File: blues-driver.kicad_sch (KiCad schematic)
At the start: 79 parts, among them Q1 LS844, Q10 BC848C, Q6 BC858C, Q7 LS844, Q8 BC858C, Q9 BC848C, U3 TLV9352

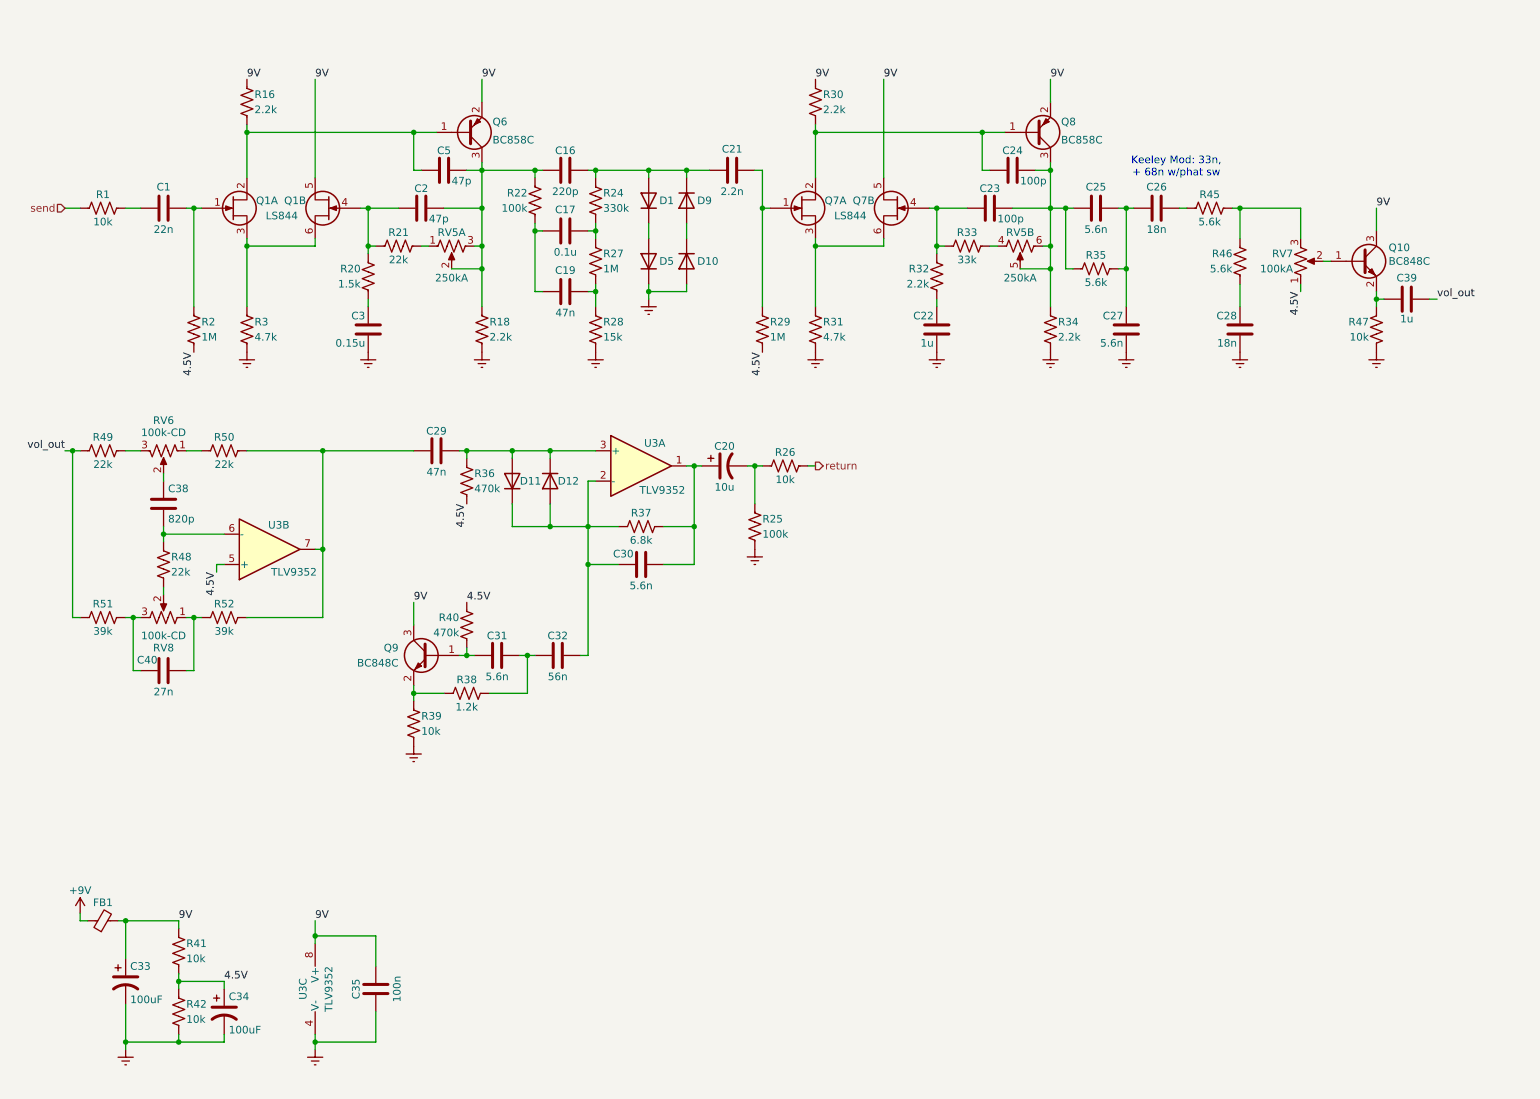
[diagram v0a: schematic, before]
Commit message: finished bd2 schematic
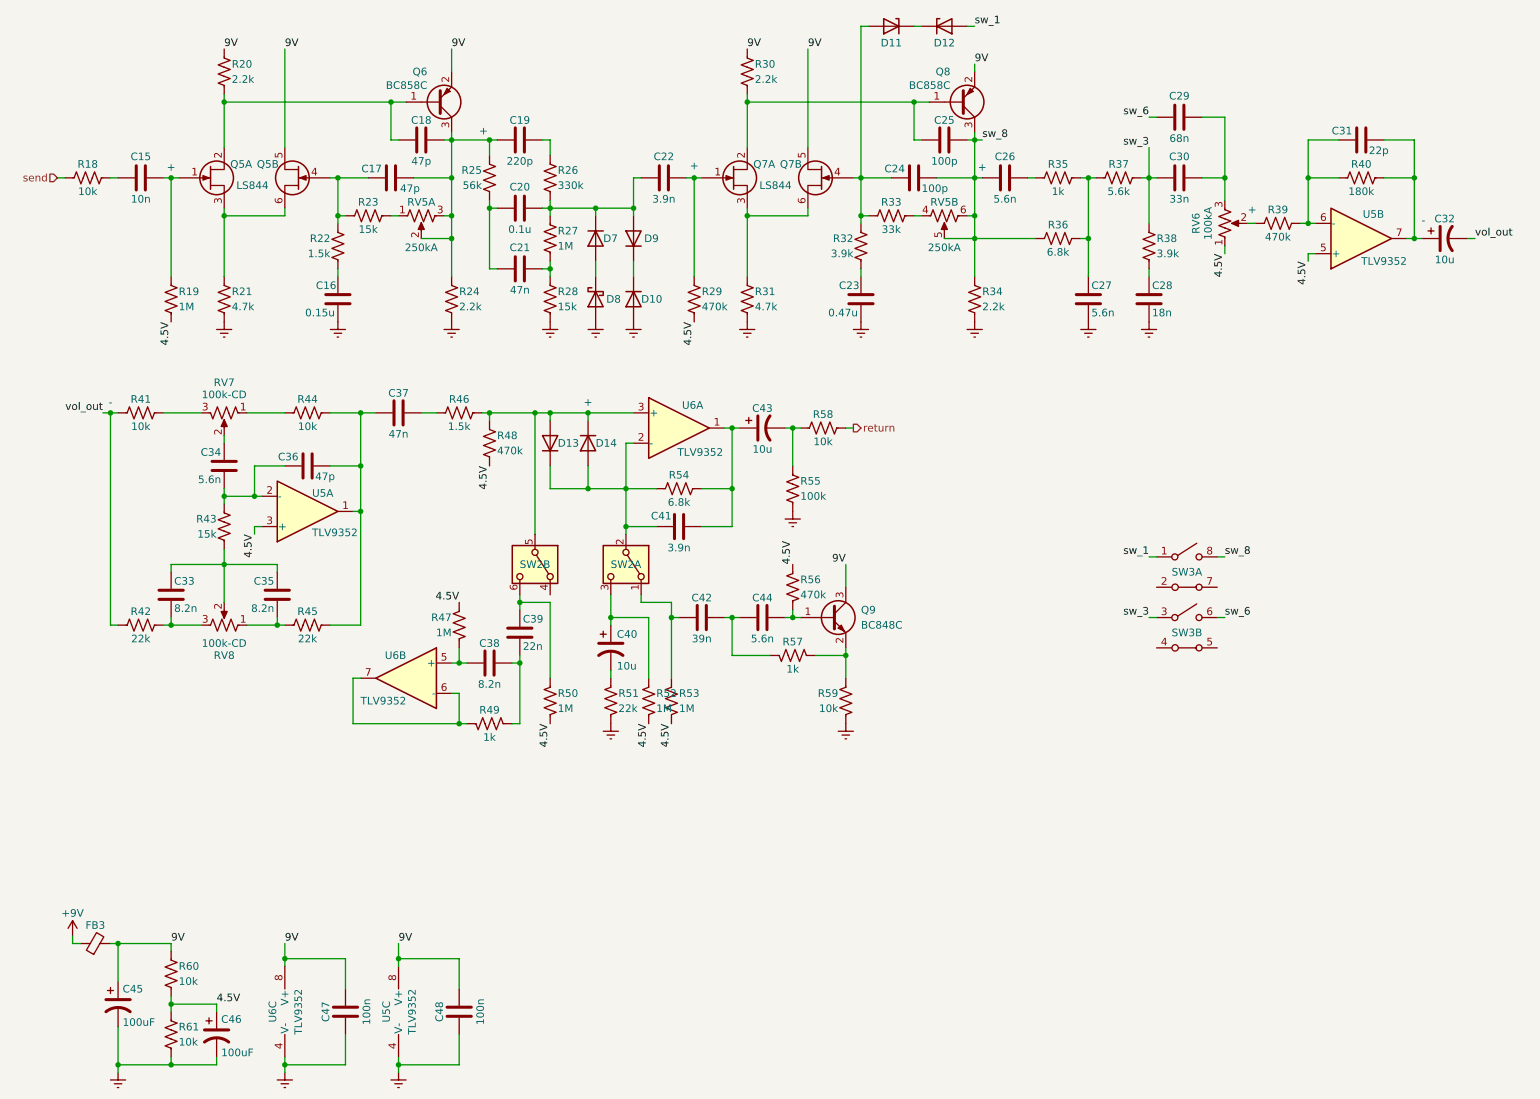
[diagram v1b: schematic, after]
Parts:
- removed C22, C39: 1u, bca-footprints:C_Film_L7.2mm_W3.5mm_P5.00mm, symbol bca-symbols:C_Film_W3.50mm
- removed C23: 100p, bca-footprints:C_Ceramic_L4.0mm_W2.5mm_P2.50mm, symbol bca-symbols:C_Ceramic
- removed C38: 820p, bca-footprints:C_Ceramic_L4.0mm_W2.5mm_P2.50mm, symbol bca-symbols:C_Ceramic
- removed C40: 27n, bca-footprints:C_Film_L7.2mm_W2.5mm_P5.00mm, symbol bca-symbols:C_Film_W2.50mm
- removed C5: 47p, bca-footprints:C_Ceramic_L4.0mm_W2.5mm_P2.50mm, symbol bca-symbols:C_Ceramic
- removed Q1: LS844, Package_TO_SOT_SMD:SOT-23-6_Handsoldering, symbol bca-symbols:LS84x_SOT23
- removed Q10: BC848C, symbol Transistor_BJT:Q_NPN_BEC
- removed R16, R18: 2.2k, bca-footprints:R_L3.6mm_D1.6mm_P5.00mm_Horizontal, symbol bca-symbols:R
- removed R3: 4.7k, bca-footprints:R_L3.6mm_D1.6mm_P5.00mm_Horizontal, symbol bca-symbols:R
- removed R48: 22k, bca-footprints:R_L3.6mm_D1.6mm_P5.00mm_Horizontal, symbol bca-symbols:R
- added C18, C36: 47p, bca-footprints:C_Ceramic_L4.0mm_W2.5mm_P2.50mm, symbol bca-symbols:C_Ceramic
- added C23: 0.47u, bca-footprints:C_Film_L7.2mm_W3.5mm_P5.00mm, symbol bca-symbols:C_Film_W3.50mm
- added C25: 100p, bca-footprints:C_Ceramic_L4.0mm_W2.5mm_P2.50mm, symbol bca-symbols:C_Ceramic
- added C29: 68n, bca-footprints:C_Film_L7.2mm_W2.5mm_P5.00mm, symbol bca-symbols:C_Film_W2.50mm
- added C31: 22p, bca-footprints:C_Ceramic_L4.0mm_W2.5mm_P2.50mm, symbol bca-symbols:C_Ceramic
- added C32, C40: 10u, bca-footprints:CP_Radial_D4.0mm_P1.50mm, symbol bca-symbols:CP_Audio
- added C33, C35, C38: 8.2n, bca-footprints:C_Film_L7.2mm_W2.5mm_P5.00mm, symbol bca-symbols:C_Film_W2.50mm
- added C34: 5.6n, bca-footprints:C_Film_L7.2mm_W2.5mm_P5.00mm, symbol bca-symbols:C_Film_W2.50mm
- added C39: 22n, bca-footprints:C_Film_L7.2mm_W2.5mm_P5.00mm, symbol bca-symbols:C_Film_W2.50mm
- added C47: 100n, bca-footprints:C_Ceramic_L4.0mm_W2.5mm_P2.50mm, symbol bca-symbols:C_Ceramic
- added D11, D12: 3v3 Zener, symbol Device:D_Zener
- added Q5: LS844, Package_TO_SOT_SMD:SOT-23-6_Handsoldering, symbol bca-symbols:LS84x_SOT23
- added R21: 4.7k, bca-footprints:R_L3.6mm_D1.6mm_P5.00mm_Horizontal, symbol bca-symbols:R
- added R22: 1.5k, bca-footprints:R_L3.6mm_D1.6mm_P5.00mm_Horizontal, symbol bca-symbols:R
- added R24: 2.2k, bca-footprints:R_L3.6mm_D1.6mm_P5.00mm_Horizontal, symbol bca-symbols:R
- added R35, R49: 1k, bca-footprints:R_L3.6mm_D1.6mm_P5.00mm_Horizontal, symbol bca-symbols:R
- added R38: 3.9k, bca-footprints:R_L3.6mm_D1.6mm_P5.00mm_Horizontal, symbol bca-symbols:R
- added R39: 470k, bca-footprints:R_L3.6mm_D1.6mm_P5.00mm_Horizontal, symbol bca-symbols:R
- added R40: 180k, bca-footprints:R_L3.6mm_D1.6mm_P5.00mm_Horizontal, symbol bca-symbols:R
- added R43: 15k, bca-footprints:R_L3.6mm_D1.6mm_P5.00mm_Horizontal, symbol bca-symbols:R
- added R50, R52, R53: 1M, bca-footprints:R_L3.6mm_D1.6mm_P5.00mm_Horizontal, symbol bca-symbols:R
- added R51: 22k, bca-footprints:R_L3.6mm_D1.6mm_P5.00mm_Horizontal, symbol bca-symbols:R
- added SW2: SW_DPDT_x2, symbol Switch:SW_DPDT_x2
- added SW3: SW_DIP_SPDT_2pos, symbol bca-symbols:SW_DIP_SPDT_2pos
- added U5: TLV9352, Package_SO:SOIC-8_3.9x4.9mm_P1.27mm, symbol Amplifier_Operational:TLV9302xD
- C15: renamed from C1; value 22n -> 10n
- C22: renamed from C21; value 2.2n -> 3.9n
- C30: renamed from C26; value 18n -> 33n
- C41: renamed from C30; value 5.6n -> 3.9n
- C42: renamed from C32; value 56n -> 39n
- D8: renamed from D5; value 1N4148 -> 1N5711; symbol Device:D -> Device:D_Schottky
- R20: value 1.5k -> 2.2k
- R23: renamed from R21; value 22k -> 15k
- R25: renamed from R22; value 100k -> 56k
- R29: value 1M -> 470k
- R32: value 2.2k -> 3.9k
- R36: renamed from R35; value 5.6k -> 6.8k
- R41: renamed from R49; value 22k -> 10k
- R42: renamed from R51; value 39k -> 22k
- R44: renamed from R50; value 22k -> 10k
- R45: renamed from R52; value 39k -> 22k
- R46: value 5.6k -> 1.5k
- R47: value 10k -> 1M
- R57: renamed from R38; value 1.2k -> 1k
- renumbered C3 to C16, C2 to C17, C16 to C19, C17 to C20, C19 to C21, C25 to C26, C29 to C37, C20 to C43, C31 to C44, C33 to C45, C34 to C46, C35 to C48, D11 to D13, D12 to D14, D9 to D7, D1 to D9, FB1 to FB3, R1 to R18, R2 to R19, R24 to R26, R45 to R37, R36 to R48, R37 to R54, R25 to R55, R40 to R56, R26 to R58, R39 to R59, R41 to R60, R42 to R61, RV7 to RV6, RV6 to RV7, U3 to U6
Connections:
- net 4.5V: now also R47.2, R50.1, R52.1, R53.1, U5.3 (+), U5.5 (+); no longer U6.5 (+)
- net 9V: now also R20.2, C47.1, Q5.5 (D2), U5.8 (V+)
- net Earth: now also D8.2 (A), C23.2, C47.2, R21.1, R24.1, R51.1, U5.4 (V-); no longer D8.1 (K), R47.1
- net vol_out: now also C32.2
- net at C41.1, D13.1 (K), D14.2 (A)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: now also SW2.2 (B); no longer C42.1
- net at D13.2 (A), D14.1 (K), R48.2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: now also R46.2, SW2.5 (B); no longer C37.2
- net at C17.1, R23.1: now also Q5.4 (G1), R22.2; no longer R20.2
- net at C20.2, R26.1, R27.2: now also C22.1, D7.1 (K), D9.2 (A)
- net at C17.2, C19.1, Q6.3 (C)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: now also C18.2, R24.2
- net at C15.2, R19.2: now also Q5.1 (G1)
- net at R42.2, RV8.3: now also C33.1
- net at C28.2: now also R38.1; no longer R46.1
- net at R45.1, RV8.1: now also C35.1
- net at C37.1, R44.2, R45.2: now also C36.2, U5.1; no longer U6.7
- net at Q6.1 (B): now also R20.1, C18.1, Q5.2 (D1)
- net at RV8.2: now also C33.2, C35.2, R43.1
- net at R32.1: now also C23.1
- net at Q7.4 (G1), R32.2, R33.1: now also C24.1, D11.2 (A)
- net at C16.1: now also R22.1; no longer R20.1
- net at RV6.2: now also R39.1
- net at Q7.2 (D1), Q8.1 (B), R30.1: now also C25.1; no longer C24.1
- net at C27.2, R36.2: now also R37.1, R35.2; no longer C26.2, C30.1
- net at C30.2: now also RV6.3, C29.2; no longer R37.1
- net sw_8: now reaches C24.2, C26.1, Q8.3 (C), R34.2, R36.1, RV5.5, RV5.6
- net sw_8: now also C25.2, SW3.8 (A)
- net at U6.6 (-): now also U6.7, R49.2
- net at RV7.2: now also C34.2
- net at D10.1 (K): now also D9.1 (K); no longer D7.2 (A)
- new net: Q5.3 (S1), Q5.6 (S1), R21.2
- new net: C26.2, R35.1
- new net: C19.2, R26.2
- new net: C38.1, R47.1, U6.5 (+)
- new net: C42.1, R53.2, SW2.1 (A)
- new net: C40.1, R52.2, SW2.3 (C)
- new net: C40.2, R51.2
- new net: C37.2, R46.1
- new net: D11.1 (K), D12.1 (K)
- new net: C38.2, C39.1, R49.1
- new net: C34.1, C36.1, R43.2, U5.2 (-)
- new net: C31.2, C32.1, R40.2, U5.7
- new net: C31.1, R39.2, R40.1, U5.6 (-)
- new net: D7.2 (A), D8.1 (K)
- new net: C39.2, R50.2, SW2.6 (C)
- new net sw_1: D12.2 (A), SW3.1 (C)
- new net sw_3: C30.1, R37.2, R38.2, SW3.3 (C)
- new net sw_6: C29.1, SW3.6 (A)
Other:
- note added: "+"
- note added: "-"
- note removed: "Keeley Mod: 33n, + 68n w/phat sw"
- moved on the sheet: C15, C16, C17, C19, C20, C21, C22, C26, C28, C30, C37, C41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
